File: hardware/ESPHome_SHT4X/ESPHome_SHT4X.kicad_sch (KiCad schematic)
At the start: 15 parts, among them SW2 SW_Push, SW3 SW_Push, U1 ESP32-C6-WROOM-1-N8

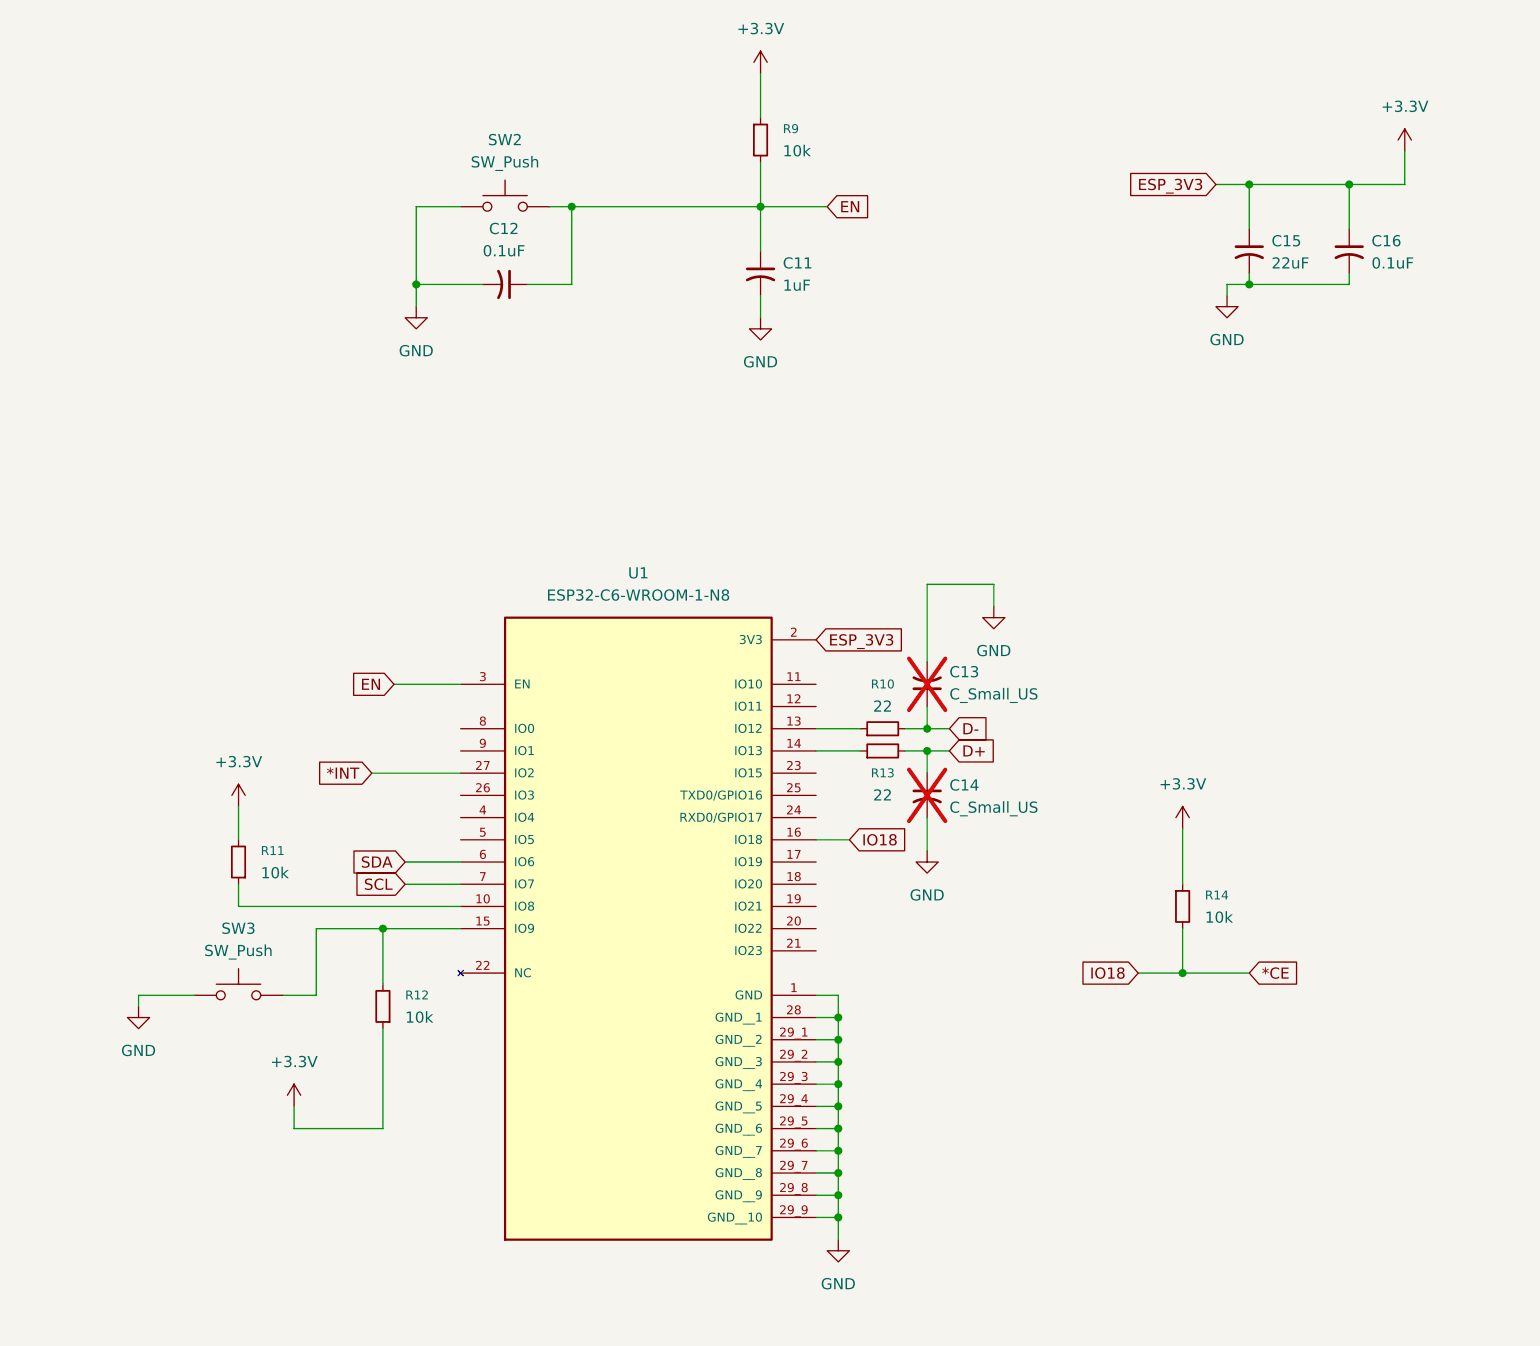
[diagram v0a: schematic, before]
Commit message: Finishing touches on schematic, started on PCB Design
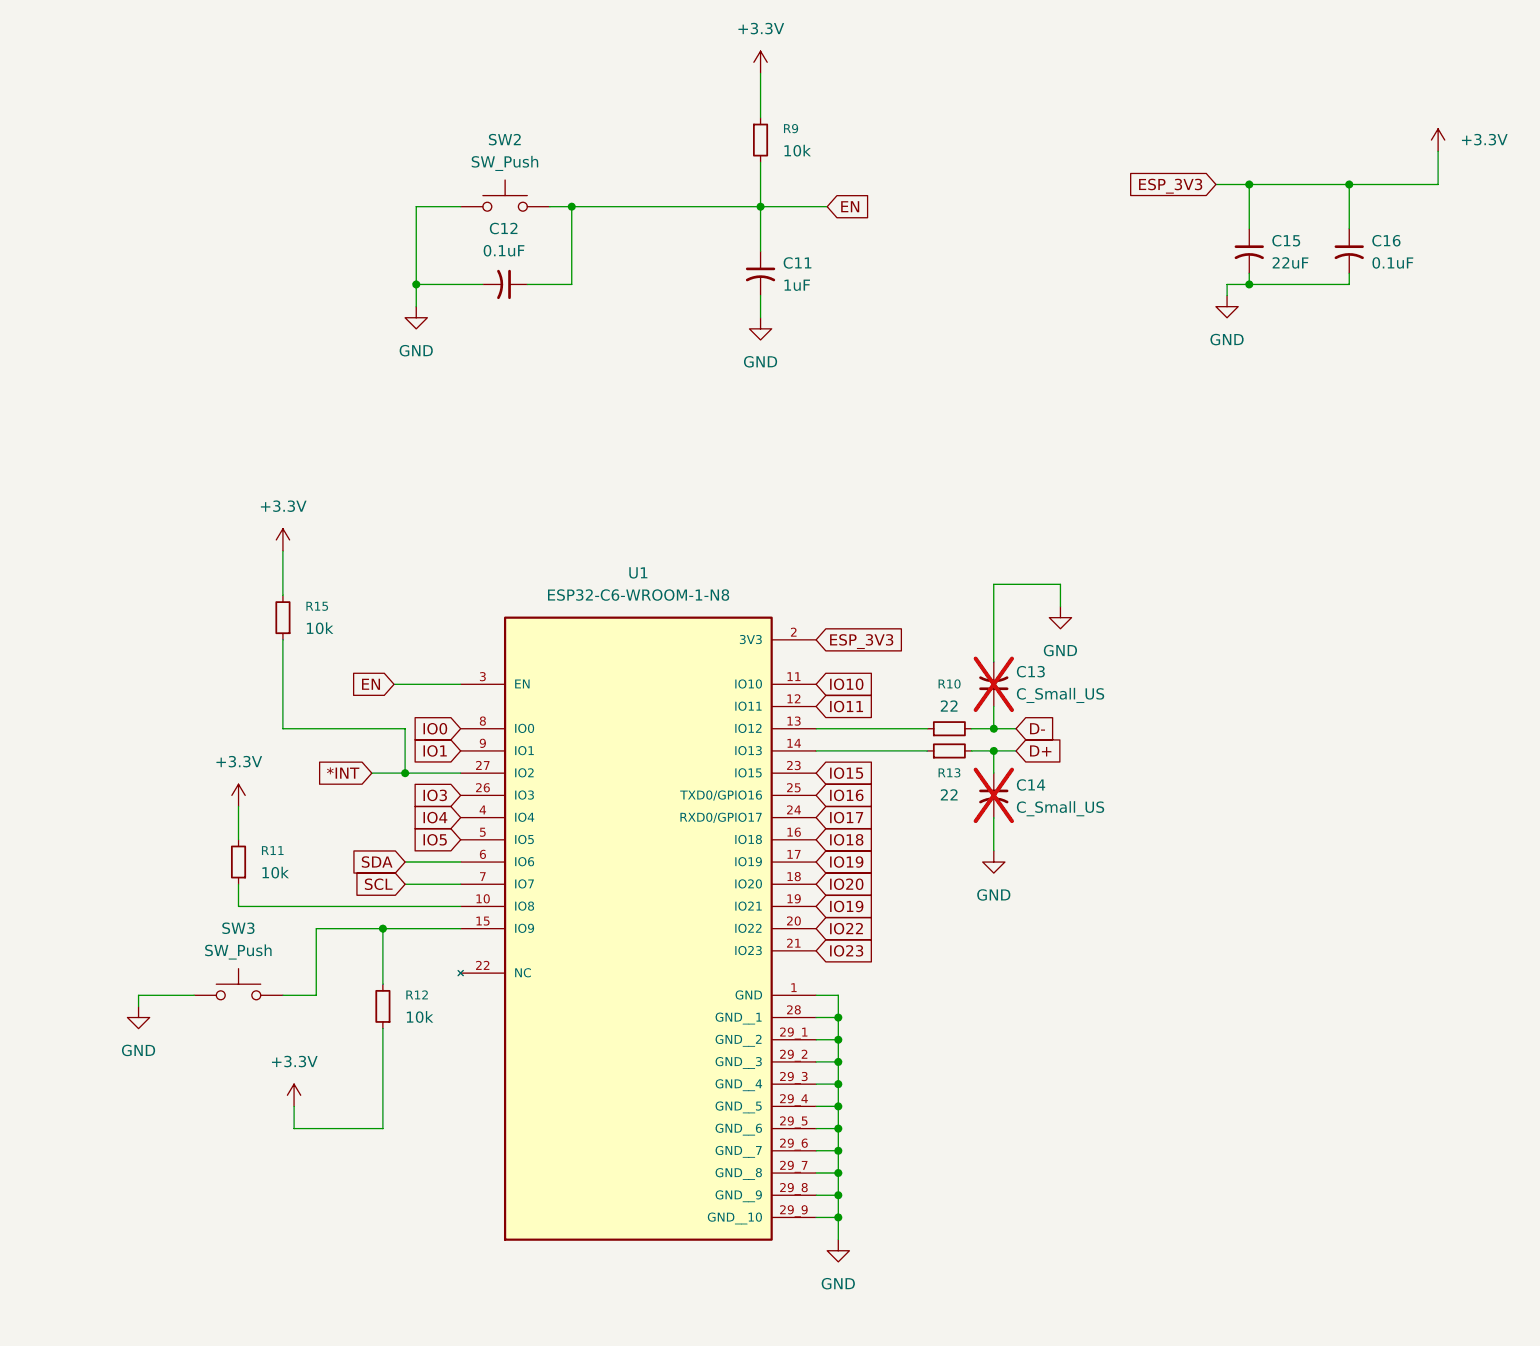
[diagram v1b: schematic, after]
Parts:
- removed R14: 10k, Package_DIP:DIP-8_W7.62mm, symbol Device:R_Small
- added R15: 10k, Resistor_SMD:R_1206_3216Metric_Pad1.30x1.75mm_HandSolder, symbol Device:R_Small
- C11, C12: footprint (none) -> Capacitor_SMD:C_1206_3216Metric_Pad1.33x1.80mm_HandSolder
- C13, C14, C15, C16: footprint LED_SMD:LED_Kingbright_APFA3010_3x1.5mm_Horizontal -> Capacitor_SMD:C_1206_3216Metric_Pad1.33x1.80mm_HandSolder
- R10, R11, R12, R13, R9: footprint Package_DIP:DIP-8_W7.62mm -> Resistor_SMD:R_1206_3216Metric_Pad1.30x1.75mm_HandSolder
- SW2, SW3: footprint Package_DIP:DIP-24_W7.62mm -> Library:SW_TS02-66-43-BK-100-SCR-D
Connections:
- net *INT: now also R15.1
- net +3.3V: now also R15.2
- net IO10: now reaches U1.11 (IO10)
- net IO11: now reaches U1.12 (IO11)
- net IO19: now reaches U1.17 (IO19)
- net IO19: now also U1.19 (IO21)
- net IO20: now reaches U1.18 (IO20)
- net IO22: now reaches U1.20 (IO22)
- net IO23: now reaches U1.21 (IO23)
- net IO15: now reaches U1.23 (IO15)
- net IO17: now reaches U1.24 (RXD0/GPIO17)
- net IO16: now reaches U1.25 (TXD0/GPIO16)
- net IO3: now reaches U1.26 (IO3)
- net IO4: now reaches U1.4 (IO4)
- net IO5: now reaches U1.5 (IO5)
- net IO0: now reaches U1.8 (IO0)
- net IO1: now reaches U1.9 (IO1)
- net *CE renamed IO18
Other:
- moved on the sheet: C13, C14, R10, R13

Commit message: Making progress
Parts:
- C11, C12, C13, C14, C15, C16: footprint Capacitor_SMD:C_1206_3216Metric_Pad1.33x1.80mm_HandSolder -> Capacitor_SMD:C_01005_0402Metric_Pad0.57x0.30mm_HandSolder
- R10, R13: footprint Resistor_SMD:R_1206_3216Metric_Pad1.30x1.75mm_HandSolder -> Inductor_SMD:L_01005_0402Metric_Pad0.57x0.30mm_HandSolder
- R11, R12, R15, R9: footprint Resistor_SMD:R_1206_3216Metric_Pad1.30x1.75mm_HandSolder -> Resistor_SMD:R_01005_0402Metric_Pad0.57x0.30mm_HandSolder
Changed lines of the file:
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@@
 			)
 		)
-		(property "Footprint" "Capacitor_SMD:C_1206_3216Metric_Pad1.33x1.80mm_HandSolder"
+		(property "Footprint" "Capacitor_SMD:C_01005_0402Metric_Pad0.57x0.30mm_HandSolder"
 			(at 127 116.84 0)
 			(hide yes)
@@
 			)
 		)
-		(property "Footprint" "Resistor_SMD:R_1206_3216Metric_Pad1.30x1.75mm_HandSolder"
+		(property "Footprint" "Resistor_SMD:R_01005_0402Metric_Pad0.57x0.30mm_HandSolder"
 			(at 40.64 124.46 0)
 			(hide yes)
@@
 			)
 		)
-		(property "Footprint" "Resistor_SMD:R_1206_3216Metric_Pad1.30x1.75mm_HandSolder"
+		(property "Footprint" "Inductor_SMD:L_01005_0402Metric_Pad0.57x0.30mm_HandSolder"
 			(at 121.92 109.22 0)
 			(hide yes)
@@
 			)
 		)
-		(property "Footprint" "Resistor_SMD:R_1206_3216Metric_Pad1.30x1.75mm_HandSolder"
+		(property "Footprint" "Resistor_SMD:R_01005_0402Metric_Pad0.57x0.30mm_HandSolder"
 			(at 57.15 140.97 0)
 			(hide yes)
@@
 			)
 		)
-		(property "Footprint" "Capacitor_SMD:C_1206_3216Metric_Pad1.33x1.80mm_HandSolder"
+		(property "Footprint" "Capacitor_SMD:C_01005_0402Metric_Pad0.57x0.30mm_HandSolder"
 			(at 156.21 54.61 0)
 			(hide yes)
@@
 			)
 		)
-		(property "Footprint" "Capacitor_SMD:C_1206_3216Metric_Pad1.33x1.80mm_HandSolder"
+		(property "Footprint" "Capacitor_SMD:C_01005_0402Metric_Pad0.57x0.30mm_HandSolder"
 			(at 100.33 57.15 0)
 			(hide yes)
@@
 			)
 		)
-		(property "Footprint" "Capacitor_SMD:C_1206_3216Metric_Pad1.33x1.80mm_HandSolder"
+		(property "Footprint" "Capacitor_SMD:C_01005_0402Metric_Pad0.57x0.30mm_HandSolder"
 			(at 127 104.14 0)
 			(hide yes)
@@
 			)
 		)
-		(property "Footprint" "Resistor_SMD:R_1206_3216Metric_Pad1.30x1.75mm_HandSolder"
+		(property "Footprint" "Resistor_SMD:R_01005_0402Metric_Pad0.57x0.30mm_HandSolder"
 			(at 45.72 96.52 0)
 			(hide yes)
@@
 			)
 		)
-		(property "Footprint" "Resistor_SMD:R_1206_3216Metric_Pad1.30x1.75mm_HandSolder"
+		(property "Footprint" "Inductor_SMD:L_01005_0402Metric_Pad0.57x0.30mm_HandSolder"
 			(at 121.92 111.76 0)
 			(hide yes)
@@
 			)
 		)
-		(property "Footprint" "Capacitor_SMD:C_1206_3216Metric_Pad1.33x1.80mm_HandSolder"
+		(property "Footprint" "Capacitor_SMD:C_01005_0402Metric_Pad0.57x0.30mm_HandSolder"
 			(at 71.12 58.42 0)
 			(hide yes)
@@
 			)
 		)
-		(property "Footprint" "Capacitor_SMD:C_1206_3216Metric_Pad1.33x1.80mm_HandSolder"
+		(property "Footprint" "Capacitor_SMD:C_01005_0402Metric_Pad0.57x0.30mm_HandSolder"
 			(at 167.64 54.61 0)
 			(hide yes)
@@
 			)
 		)
-		(property "Footprint" "Resistor_SMD:R_1206_3216Metric_Pad1.30x1.75mm_HandSolder"
+		(property "Footprint" "Resistor_SMD:R_01005_0402Metric_Pad0.57x0.30mm_HandSolder"
 			(at 100.33 41.91 0)
 			(hide yes)

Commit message: making progress
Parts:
- C11, C12, C13, C14, C15, C16: footprint Capacitor_SMD:C_01005_0402Metric_Pad0.57x0.30mm_HandSolder -> Capacitor_SMD:C_0201_0603Metric_Pad0.64x0.40mm_HandSolder
- R10, R13: footprint Inductor_SMD:L_01005_0402Metric_Pad0.57x0.30mm_HandSolder -> Inductor_SMD:L_0201_0603Metric_Pad0.64x0.40mm_HandSolder
- R11, R12, R15, R9: footprint Resistor_SMD:R_01005_0402Metric_Pad0.57x0.30mm_HandSolder -> Resistor_SMD:R_0201_0603Metric_Pad0.64x0.40mm_HandSolder
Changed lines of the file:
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@@
 			)
 		)
-		(property "Footprint" "Capacitor_SMD:C_01005_0402Metric_Pad0.57x0.30mm_HandSolder"
+		(property "Footprint" "Capacitor_SMD:C_0201_0603Metric_Pad0.64x0.40mm_HandSolder"
 			(at 127 116.84 0)
 			(hide yes)
@@
 			)
 		)
-		(property "Footprint" "Resistor_SMD:R_01005_0402Metric_Pad0.57x0.30mm_HandSolder"
+		(property "Footprint" "Resistor_SMD:R_0201_0603Metric_Pad0.64x0.40mm_HandSolder"
 			(at 40.64 124.46 0)
 			(hide yes)
@@
 			)
 		)
-		(property "Footprint" "Inductor_SMD:L_01005_0402Metric_Pad0.57x0.30mm_HandSolder"
+		(property "Footprint" "Inductor_SMD:L_0201_0603Metric_Pad0.64x0.40mm_HandSolder"
 			(at 121.92 109.22 0)
 			(hide yes)
@@
 			)
 		)
-		(property "Footprint" "Resistor_SMD:R_01005_0402Metric_Pad0.57x0.30mm_HandSolder"
+		(property "Footprint" "Resistor_SMD:R_0201_0603Metric_Pad0.64x0.40mm_HandSolder"
 			(at 57.15 140.97 0)
 			(hide yes)
@@
 			)
 		)
-		(property "Footprint" "Capacitor_SMD:C_01005_0402Metric_Pad0.57x0.30mm_HandSolder"
+		(property "Footprint" "Capacitor_SMD:C_0201_0603Metric_Pad0.64x0.40mm_HandSolder"
 			(at 156.21 54.61 0)
 			(hide yes)
@@
 			)
 		)
-		(property "Footprint" "Capacitor_SMD:C_01005_0402Metric_Pad0.57x0.30mm_HandSolder"
+		(property "Footprint" "Capacitor_SMD:C_0201_0603Metric_Pad0.64x0.40mm_HandSolder"
 			(at 100.33 57.15 0)
 			(hide yes)
@@
 			)
 		)
-		(property "Footprint" "Capacitor_SMD:C_01005_0402Metric_Pad0.57x0.30mm_HandSolder"
+		(property "Footprint" "Capacitor_SMD:C_0201_0603Metric_Pad0.64x0.40mm_HandSolder"
 			(at 127 104.14 0)
 			(hide yes)
@@
 			)
 		)
-		(property "Footprint" "Resistor_SMD:R_01005_0402Metric_Pad0.57x0.30mm_HandSolder"
+		(property "Footprint" "Resistor_SMD:R_0201_0603Metric_Pad0.64x0.40mm_HandSolder"
 			(at 45.72 96.52 0)
 			(hide yes)
@@
 			)
 		)
-		(property "Footprint" "Inductor_SMD:L_01005_0402Metric_Pad0.57x0.30mm_HandSolder"
+		(property "Footprint" "Inductor_SMD:L_0201_0603Metric_Pad0.64x0.40mm_HandSolder"
 			(at 121.92 111.76 0)
 			(hide yes)
@@
 			)
 		)
-		(property "Footprint" "Capacitor_SMD:C_01005_0402Metric_Pad0.57x0.30mm_HandSolder"
+		(property "Footprint" "Capacitor_SMD:C_0201_0603Metric_Pad0.64x0.40mm_HandSolder"
 			(at 71.12 58.42 0)
 			(hide yes)
@@
 			)
 		)
-		(property "Footprint" "Capacitor_SMD:C_01005_0402Metric_Pad0.57x0.30mm_HandSolder"
+		(property "Footprint" "Capacitor_SMD:C_0201_0603Metric_Pad0.64x0.40mm_HandSolder"
 			(at 167.64 54.61 0)
 			(hide yes)
@@
 			)
 		)
-		(property "Footprint" "Resistor_SMD:R_01005_0402Metric_Pad0.57x0.30mm_HandSolder"
+		(property "Footprint" "Resistor_SMD:R_0201_0603Metric_Pad0.64x0.40mm_HandSolder"
 			(at 100.33 41.91 0)
 			(hide yes)

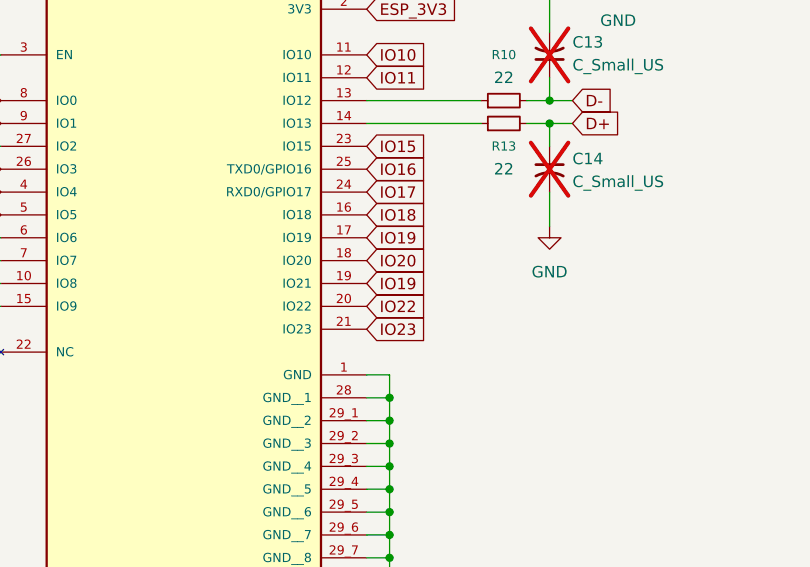
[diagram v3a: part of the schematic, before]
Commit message: Continued work on PCB Layout
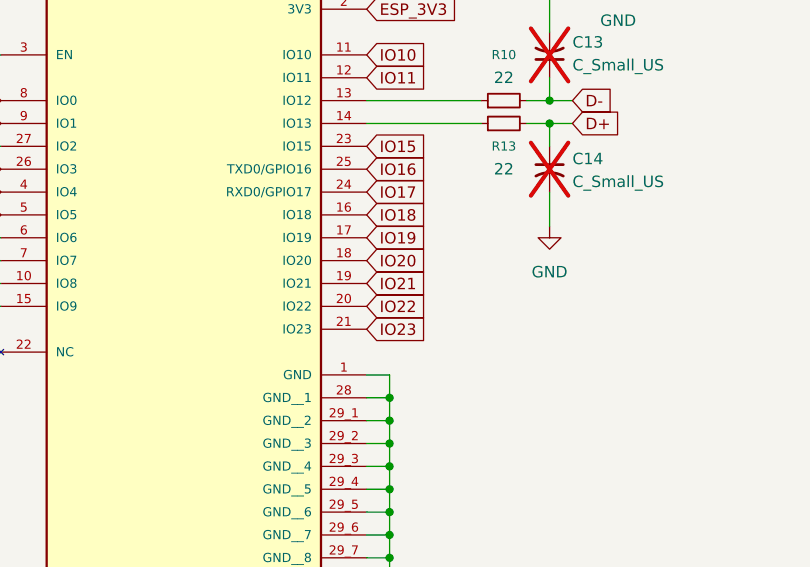
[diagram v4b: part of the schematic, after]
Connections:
- net IO19: no longer U1.19 (IO21)
- new net IO21: U1.19 (IO21)
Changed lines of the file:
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@@
 		)
 	)
-	(global_label "IO19"
+	(global_label "IO21"
 		(shape input)
 		(at 106.68 129.54 0)
